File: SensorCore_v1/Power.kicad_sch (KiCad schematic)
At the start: 11 parts, among them U3 R-78K3.3-1.0

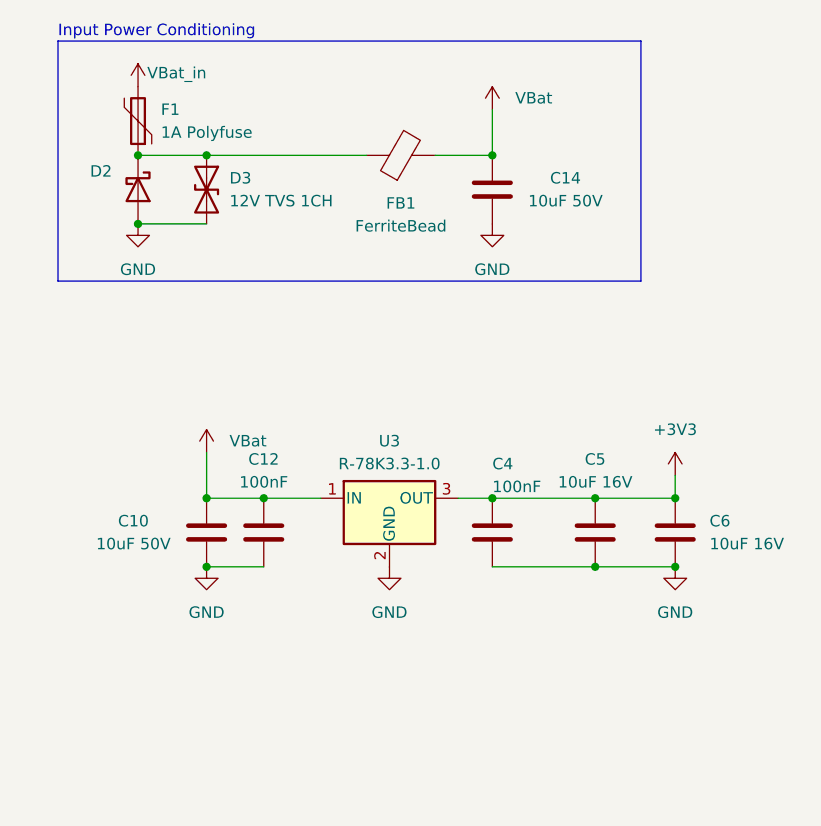
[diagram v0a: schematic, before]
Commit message: Misc. Tweaks to files
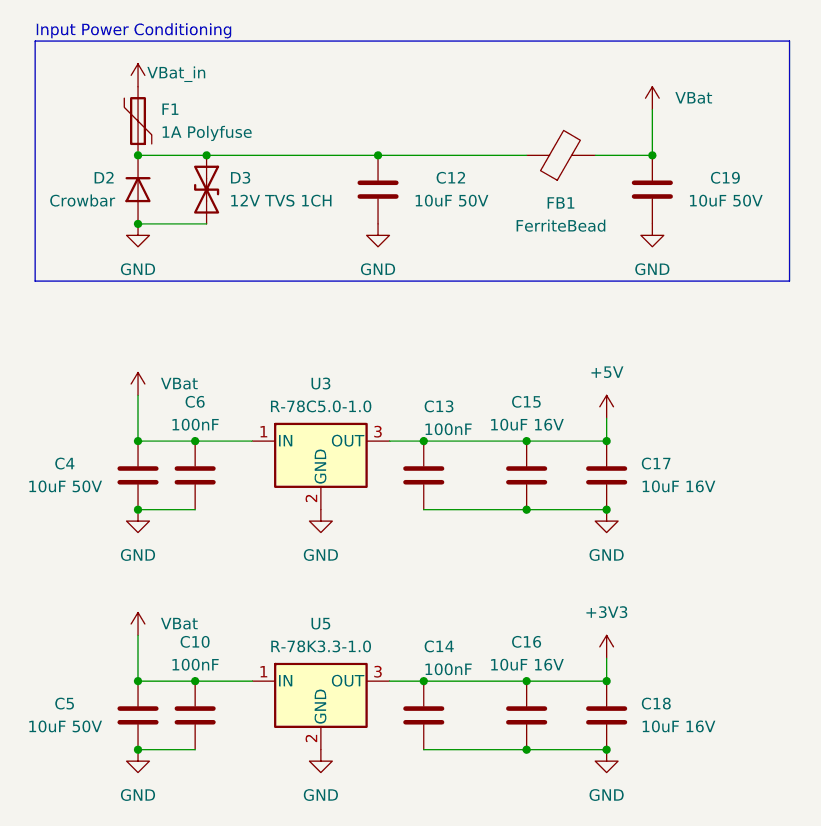
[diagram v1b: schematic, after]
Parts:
- removed D2: D_Schottky, symbol Device:D_Schottky
- added C12, C4: 10uF 50V, Capacitor_SMD:C_0805_2012Metric_Pad1.18x1.45mm_HandSolder, symbol Device:C
- added C13, C6: 100nF, Resistor_SMD:R_0603_1608Metric_Pad0.98x0.95mm_HandSolder, symbol Device:C
- added C15, C17: 10uF 16V, Capacitor_SMD:C_0805_2012Metric_Pad1.18x1.45mm_HandSolder, symbol Device:C
- added D2: Crowbar, symbol Device:D
- added U3: R-78C5.0-1.0, Converter_DCDC:Converter_DCDC_RECOM_R-78E-0.5_THT, symbol Regulator_Switching:R-78C5.0-1.0
- renumbered C12 to C10, C4 to C14, C5 to C16, C6 to C18, C14 to C19, C10 to C5, U3 to U5
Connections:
- net GND: now also C12.2, C13.1, C15.2, C17.2, C4.2, C6.1, D2.2 (A), U3.2 (GND)
- net VBat: now also C4.1, C6.2, U3.1 (IN)
- net at D3.1 (A1), F1.1, FB1.1: now also C12.1, D2.1 (K)
- new net +5V: C13.2, C15.1, C17.1, U3.3 (OUT)
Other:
- moved on the sheet: C10, C14, C16, C18, C19, C5, FB1, U5
